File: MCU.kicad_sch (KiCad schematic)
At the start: 47 parts, among them J1 SWD_LOG, Q2 BC847, SW1 SW_Push, U1 STM32F429IGTx, Y1 25MHz, Y5 32.768KHz

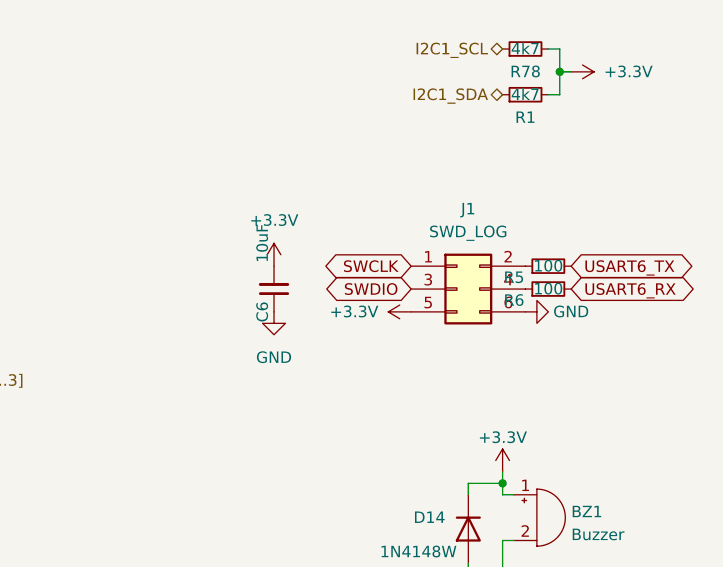
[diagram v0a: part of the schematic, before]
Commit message: None.
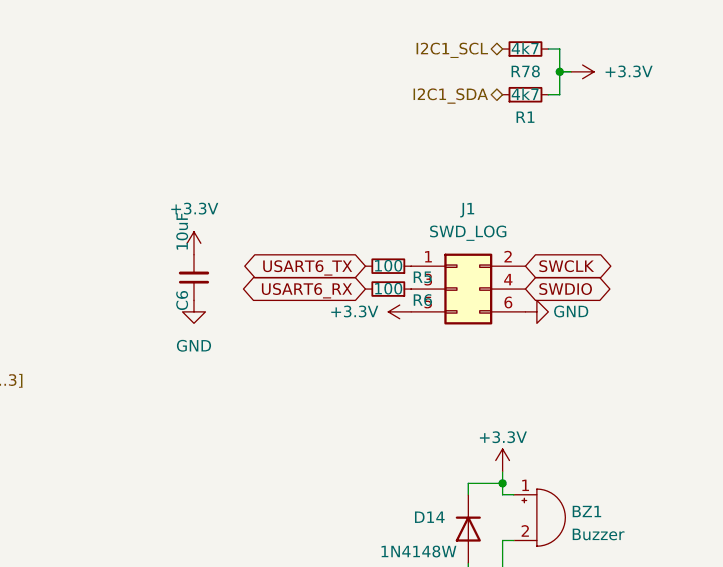
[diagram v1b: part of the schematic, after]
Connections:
- net SWCLK: now also J1.2 (Pin_2); no longer J1.1 (Pin_1)
- net SWDIO: now also J1.4 (Pin_4); no longer J1.3 (Pin_3)
- net at R6.1: now also J1.3 (Pin_3); no longer J1.4 (Pin_4)
- net at R5.1: now also J1.1 (Pin_1); no longer J1.2 (Pin_2)
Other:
- moved on the sheet: C6, R5, R6
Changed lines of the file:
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@@
     )
   )
-  (global_label "SWCLK" (shape bidirectional) (at 220.98 200.66 180) (fields_autoplaced)
-    (effects (font (size 1.27 1.27)) (justify right))
-    (property "Intersheetrefs" "${INTERSHEET_REFS}" (at 212.3379 200.7394 0)
-      (effects (font (size 1.27 1.27)) (justify right) hide)
+  (global_label "SWCLK" (shape bidirectional) (at 233.68 200.66 0) (fields_autoplaced)
+    (effects (font (size 1.27 1.27)) (justify left))
+    (property "Intersheetrefs" "${INTERSHEET_REFS}" (at 242.3221 200.7394 0)
+      (effects (font (size 1.27 1.27)) (justify left) hide)
     )
   )
@@
     )
   )
-  (global_label "SWDIO" (shape bidirectional) (at 220.98 203.2 180) (fields_autoplaced)
-    (effects (font (size 1.27 1.27)) (justify right))
-    (property "Intersheetrefs" "${INTERSHEET_REFS}" (at 212.7007 203.2794 0)
-      (effects (font (size 1.27 1.27)) (justify right) hide)
+  (global_label "SWDIO" (shape bidirectional) (at 233.68 203.2 0) (fields_autoplaced)
+    (effects (font (size 1.27 1.27)) (justify left))
+    (property "Intersheetrefs" "${INTERSHEET_REFS}" (at 241.9593 203.2794 0)
+      (effects (font (size 1.27 1.27)) (justify left) hide)
     )
   )
@@
     )
   )
-  (global_label "USART6_RX" (shape bidirectional) (at 238.76 203.2 0) (fields_autoplaced)
-    (effects (font (size 1.27 1.27)) (justify left))
-    (property "Intersheetrefs" "${INTERSHEET_REFS}" (at 0 -2.54 0)
-      (effects (font (size 1.27 1.27)) hide)
-    )
-  )
-  (global_label "USART6_TX" (shape bidirectional) (at 238.76 200.66 0) (fields_autoplaced)
-    (effects (font (size 1.27 1.27)) (justify left))
-    (property "Intersheetrefs" "${INTERSHEET_REFS}" (at 0 -2.54 0)
+  (global_label "USART6_RX" (shape bidirectional) (at 215.9 203.2 180) (fields_autoplaced)
+    (effects (font (size 1.27 1.27)) (justify right))
+    (property "Intersheetrefs" "${INTERSHEET_REFS}" (at 454.66 -2.54 0)
+      (effects (font (size 1.27 1.27)) hide)
+    )
+  )
+  (global_label "USART6_TX" (shape bidirectional) (at 215.9 200.66 180) (fields_autoplaced)
+    (effects (font (size 1.27 1.27)) (justify right))
+    (property "Intersheetrefs" "${INTERSHEET_REFS}" (at 454.66 -2.54 0)
       (effects (font (size 1.27 1.27)) hide)
     )
@@
     )
   )
-  (symbol (lib_id "Device:C_Small") (at 205.74 203.2 180) (unit 1)
-    (in_bom yes) (on_board yes) (dnp no)
-    (property "Reference" "C6" (at 204.47 205.74 90)
-      (effects (font (size 1.27 1.27)))
-    )
-    (property "Value" "10uF" (at 204.47 198.12 90)
-      (effects (font (size 1.27 1.27)))
-    )
-    (property "Footprint" "Anh_Footprints:C_1206" (at 205.74 203.2 0)
-      (effects (font (size 1.27 1.27)) hide)
-    )
-    (property "Datasheet" "~" (at 205.74 203.2 0)
+  (symbol (lib_id "Device:C_Small") (at 196.85 201.93 180) (unit 1)
+    (in_bom yes) (on_board yes) (dnp no)
+    (property "Reference" "C6" (at 195.58 204.47 90)
+      (effects (font (size 1.27 1.27)))
+    )
+    (property "Value" "10uF" (at 195.58 196.85 90)
+      (effects (font (size 1.27 1.27)))
+    )
+    (property "Footprint" "Anh_Footprints:C_1206" (at 196.85 201.93 0)
+      (effects (font (size 1.27 1.27)) hide)
+    )
+    (property "Datasheet" "~" (at 196.85 201.93 0)
       (effects (font (size 1.27 1.27)) hide)
     )
@@
     )
   )
-  (symbol (lib_id "power:+3.3V") (at 205.74 200.66 0) (mirror y) (unit 1)
+  (symbol (lib_id "power:+3.3V") (at 196.85 199.39 0) (mirror y) (unit 1)
     (in_bom yes) (on_board yes) (dnp no) (fields_autoplaced)
-    (property "Reference" "#PWR017" (at 205.74 204.47 0)
-      (effects (font (size 1.27 1.27)) hide)
-    )
-    (property "Value" "+3.3V" (at 205.74 195.58 0)
-      (effects (font (size 1.27 1.27)))
-    )
-    (property "Footprint" "" (at 205.74 200.66 0)
-      (effects (font (size 1.27 1.27)) hide)
-    )
-    (property "Datasheet" "" (at 205.74 200.66 0)
+    (property "Reference" "#PWR017" (at 196.85 203.2 0)
+      (effects (font (size 1.27 1.27)) hide)
+    )
+    (property "Value" "+3.3V" (at 196.85 194.31 0)
+      (effects (font (size 1.27 1.27)))
+    )
+    (property "Footprint" "" (at 196.85 199.39 0)
+      (effects (font (size 1.27 1.27)) hide)
+    )
+    (property "Datasheet" "" (at 196.85 199.39 0)
       (effects (font (size 1.27 1.27)) hide)
     )
@@
     )
   )
-  (symbol (lib_id "Device:R_Small") (at 236.22 203.2 90) (unit 1)
-    (in_bom yes) (on_board yes) (dnp no)
-    (property "Reference" "R6" (at 232.41 204.47 90)
-      (effects (font (size 1.27 1.27)))
-    )
-    (property "Value" "100" (at 236.22 203.2 90)
-      (effects (font (size 1.27 1.27)))
-    )
-    (property "Footprint" "Anh_Footprints:R_0603" (at 236.22 203.2 0)
-      (effects (font (size 1.27 1.27)) hide)
-    )
-    (property "Datasheet" "~" (at 236.22 203.2 0)
+  (symbol (lib_id "Device:R_Small") (at 218.44 203.2 270) (mirror x) (unit 1)
+    (in_bom yes) (on_board yes) (dnp no)
+    (property "Reference" "R6" (at 222.25 204.47 90)
+      (effects (font (size 1.27 1.27)))
+    )
+    (property "Value" "100" (at 218.44 203.2 90)
+      (effects (font (size 1.27 1.27)))
+    )
+    (property "Footprint" "Anh_Footprints:R_0603" (at 218.44 203.2 0)
+      (effects (font (size 1.27 1.27)) hide)
+    )
+    (property "Datasheet" "~" (at 218.44 203.2 0)
       (effects (font (size 1.27 1.27)) hide)
     )
@@
     )
   )
-  (symbol (lib_id "Device:R_Small") (at 236.22 200.66 90) (unit 1)
-    (in_bom yes) (on_board yes) (dnp no)
-    (property "Reference" "R5" (at 232.41 201.93 90)
-      (effects (font (size 1.27 1.27)))
-    )
-    (property "Value" "100" (at 236.22 200.66 90)
-      (effects (font (size 1.27 1.27)))
-    )
-    (property "Footprint" "Anh_Footprints:R_0603" (at 236.22 200.66 0)
-      (effects (font (size 1.27 1.27)) hide)
-    )
-    (property "Datasheet" "~" (at 236.22 200.66 0)
+  (symbol (lib_id "Device:R_Small") (at 218.44 200.66 270) (mirror x) (unit 1)
+    (in_bom yes) (on_board yes) (dnp no)
+    (property "Reference" "R5" (at 222.25 201.93 90)
+      (effects (font (size 1.27 1.27)))
+    )
+    (property "Value" "100" (at 218.44 200.66 90)
+      (effects (font (size 1.27 1.27)))
+    )
+    (property "Footprint" "Anh_Footprints:R_0603" (at 218.44 200.66 0)
+      (effects (font (size 1.27 1.27)) hide)
+    )
+    (property "Datasheet" "~" (at 218.44 200.66 0)
       (effects (font (size 1.27 1.27)) hide)
     )
@@
     )
   )
-  (symbol (lib_id "power:GND") (at 205.74 205.74 0) (mirror y) (unit 1)
+  (symbol (lib_id "power:GND") (at 196.85 204.47 0) (mirror y) (unit 1)
     (in_bom yes) (on_board yes) (dnp no) (fields_autoplaced)
-    (property "Reference" "#PWR018" (at 205.74 212.09 0)
-      (effects (font (size 1.27 1.27)) hide)
-    )
-    (property "Value" "GND" (at 205.74 210.82 0)
-      (effects (font (size 1.27 1.27)))
-    )
-    (property "Footprint" "" (at 205.74 205.74 0)
-      (effects (font (size 1.27 1.27)) hide)
-    )
-    (property "Datasheet" "" (at 205.74 205.74 0)
-      (effects (font (size 1.27 1.27)) hide)
-    )
+    (property "Reference" "#PWR018" (at 196.85 210.82 0)
+      (effects (font (size 1.27 1.27)) hide)
+    )
+    (property "Value" "GND" (at 196.85 209.55 0)
+      (effects (font (size 1.27 1.27)))
+    )
+    (property "Footprint" "" (at 196.85 204.47 0)
+      (effects (font (size 1.27 1.27)) hide)
+    )
+    (property "Datasheet" "" (at 196.85 204.47 0)
+      (effects (font (size 1.27 1.27)) hide)
+    )
